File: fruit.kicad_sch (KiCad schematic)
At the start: 7 parts, among them J1 PCB_Edge_PCI_Express_x4_Salmo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

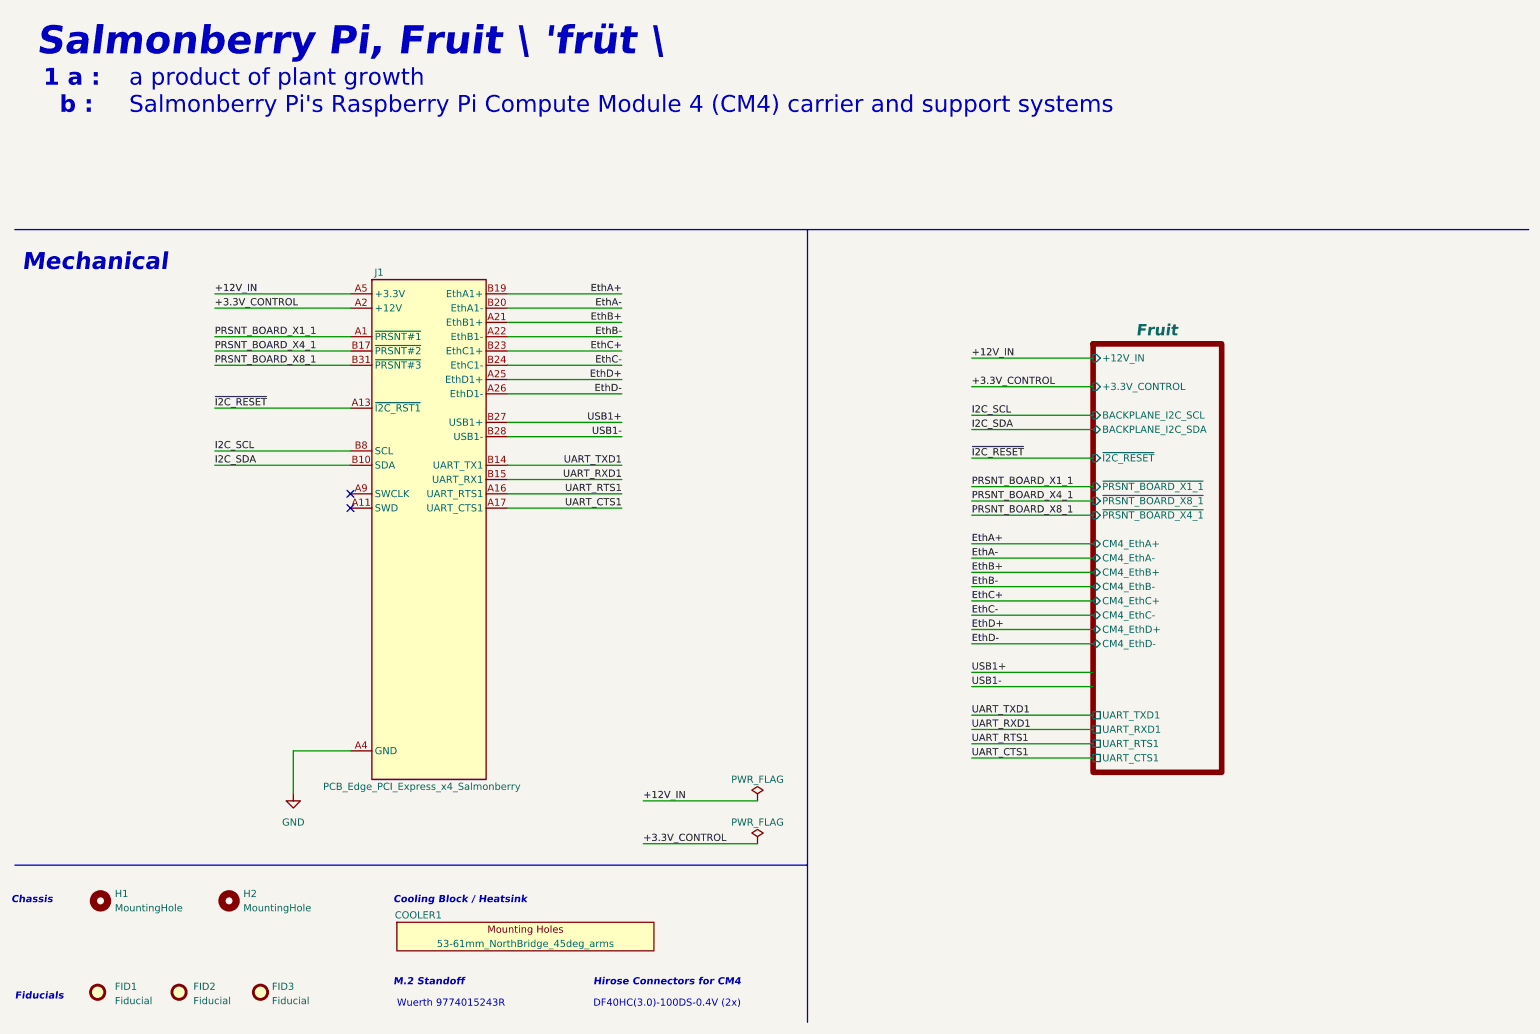
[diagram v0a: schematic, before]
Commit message: work on control logic
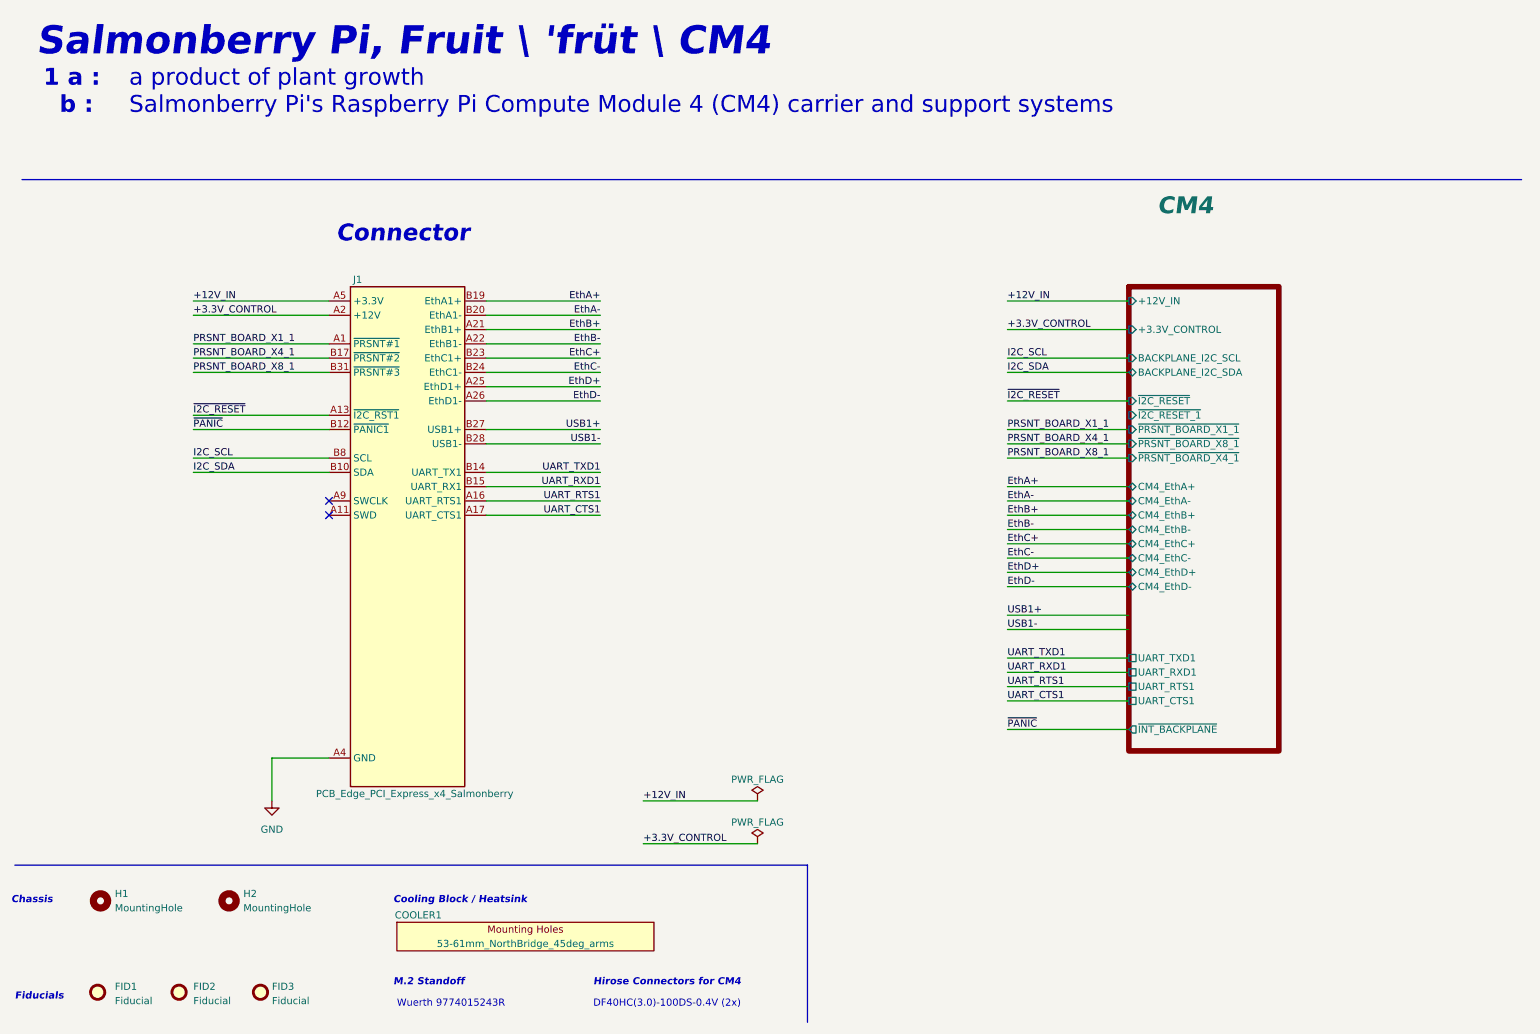
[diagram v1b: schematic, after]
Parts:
- J1: footprint Connector_PCIe_MyOwn:BUS_PCIexpress_x4_Salmonberry_reduced_shoulders -> Connector_PCIe_MyOwn:BUS_PCIexpress_x4_Salmonberry
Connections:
- net GND: no longer J1.B12 (GND)
- new net ~{PANIC}: J1.B12 (~{PANIC1})
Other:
- sheet Fruit renamed CM4
- sheet CM4 ports: added ~{I2C_RESET_1}, ~{INT_BACKPLANE}; removed none
- note added: "Connector"
- note added: "Salmonberry Pi, Fruit \ 'früt \ CM4"
- note removed: "Mechanical"
- note removed: "Salmonberry Pi, Fruit \ 'früt \"
